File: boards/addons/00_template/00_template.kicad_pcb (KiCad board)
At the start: 2 copper layers, 47 x 72 mm, 1 part, among them J1 Conn_02x15_Odd_Even

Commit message: テンプレミスの修正
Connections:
- net /GP8 renamed /GP6
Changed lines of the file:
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@@
 	(net 5 "/SPI_CS")
 	(net 6 "/GP0")
-	(net 7 "/GP8")
+	(net 7 "/GP6")
 	(net 8 "/I2C_SCL")
 	(net 9 "/GP3")
@@
 			(layers "*.Cu" "*.Mask")
 			(remove_unused_layers no)
-			(net 7 "/GP8")
+			(net 7 "/GP6")
 			(pinfunction "Pin_16")
 			(pintype "passive")

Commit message: ピン配変更
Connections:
- J1 pad 7: /SPI_MISO -> /SPI_CS
- J1 pad 8: /SPI_CS -> /SPI_MISO
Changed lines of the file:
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@@
 			(layers "*.Cu" "*.Mask")
 			(remove_unused_layers no)
-			(net 14 "/SPI_MISO")
+			(net 5 "/SPI_CS")
 			(pinfunction "Pin_7")
 			(pintype "passive")
@@
 			(layers "*.Cu" "*.Mask")
 			(remove_unused_layers no)
-			(net 5 "/SPI_CS")
+			(net 14 "/SPI_MISO")
 			(pinfunction "Pin_8")
 			(pintype "passive")

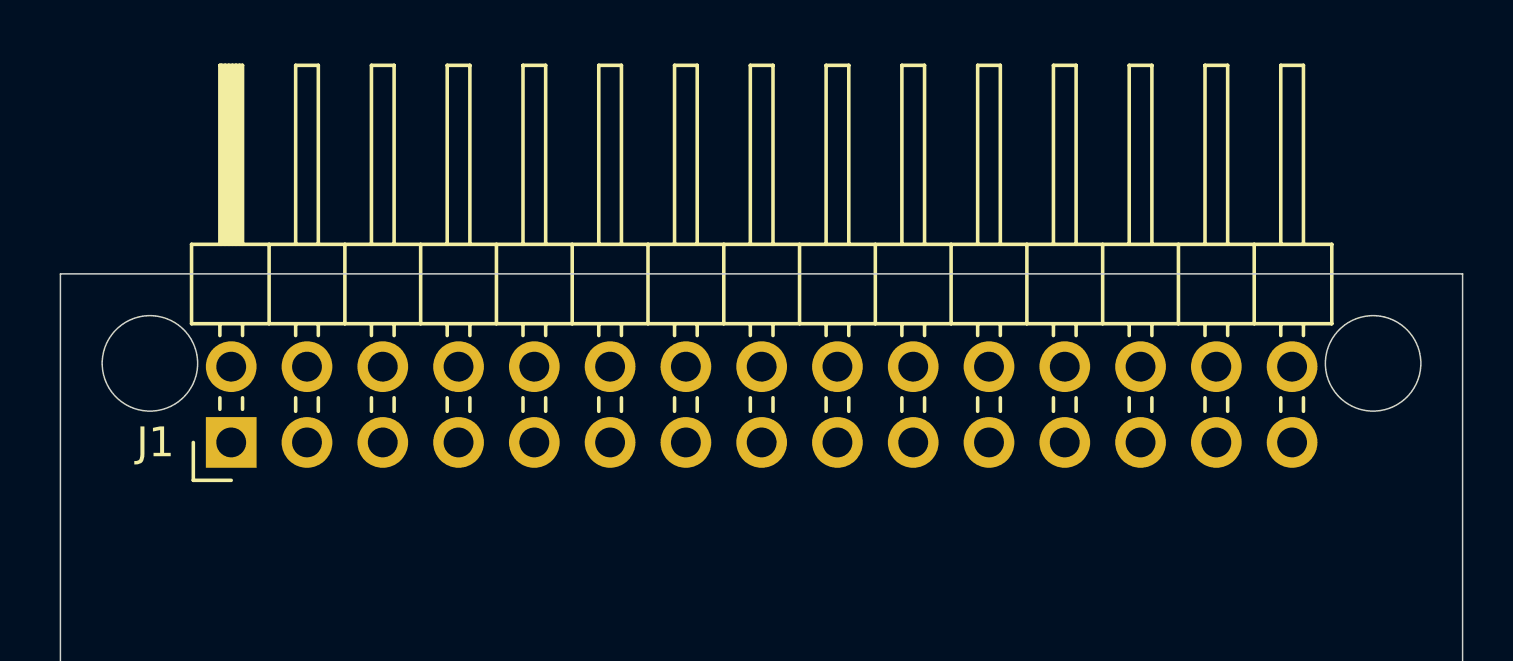
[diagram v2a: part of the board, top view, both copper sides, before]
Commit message: テンプレ修正
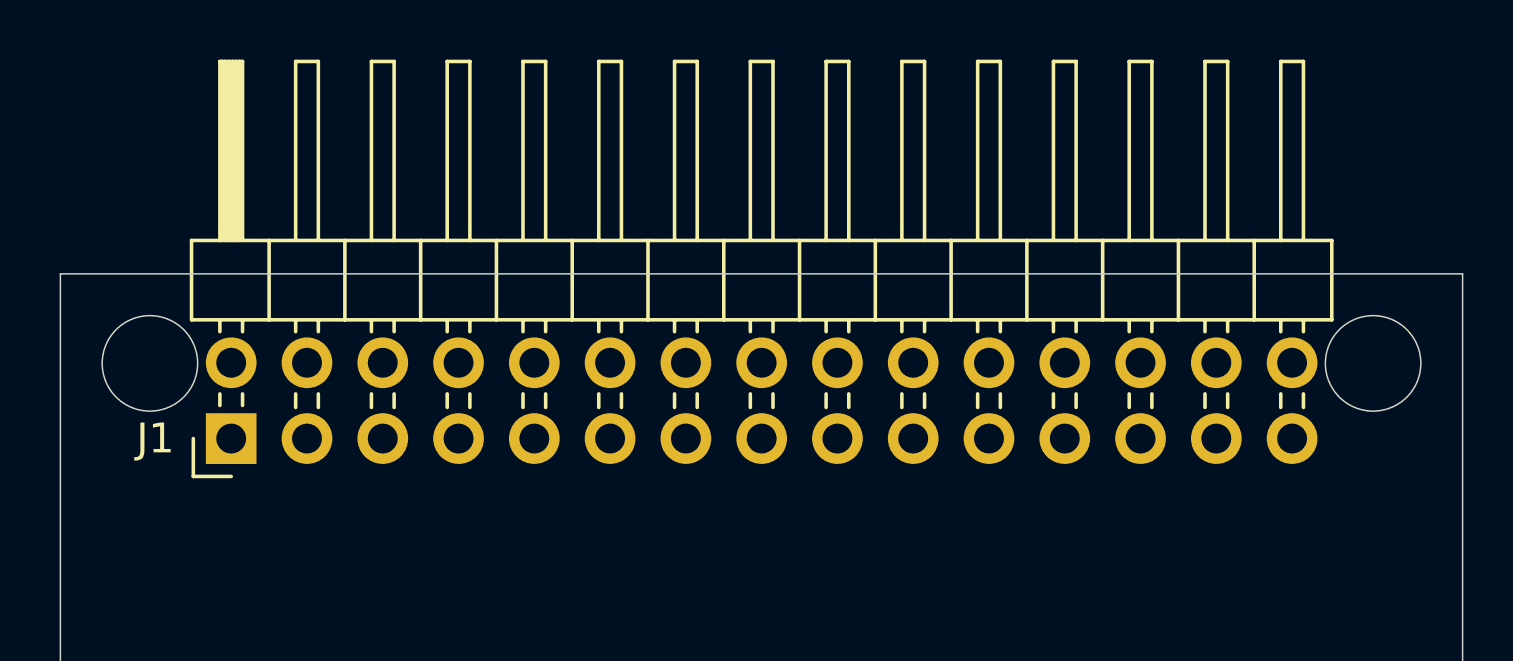
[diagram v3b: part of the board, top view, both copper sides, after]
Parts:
- moved J1 0.13 mm to (134.6, 71.1)
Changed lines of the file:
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@@
 	(footprint "Connector_PinHeader_2.54mm:PinHeader_2x15_P2.54mm_Horizontal"
 		(layer "F.Cu")
-		(at 134.625 71.25 90)
+		(at 134.625 71.12 90)
 		(descr "Through hole angled pin header, 2x15, 2.54mm pitch, 6mm pin length, double rows")
 		(tags "Through hole angled pin header THT 2x15 2.54mm double row")
